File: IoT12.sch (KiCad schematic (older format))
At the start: 98 parts, among them J1 Conn_01x04_Male, Q1 2N7002, Q2 2N7002, Q3 AOD403, SW1 Rotary encoder EC11 Plum 15mm, U1 MAX809S, U2 AT24C32, U3 INA826AID, U4 INA826AID, U5 ADS1115IDGS, U6 LM393, U7 74HC125, U8 LM2596S-ADJ

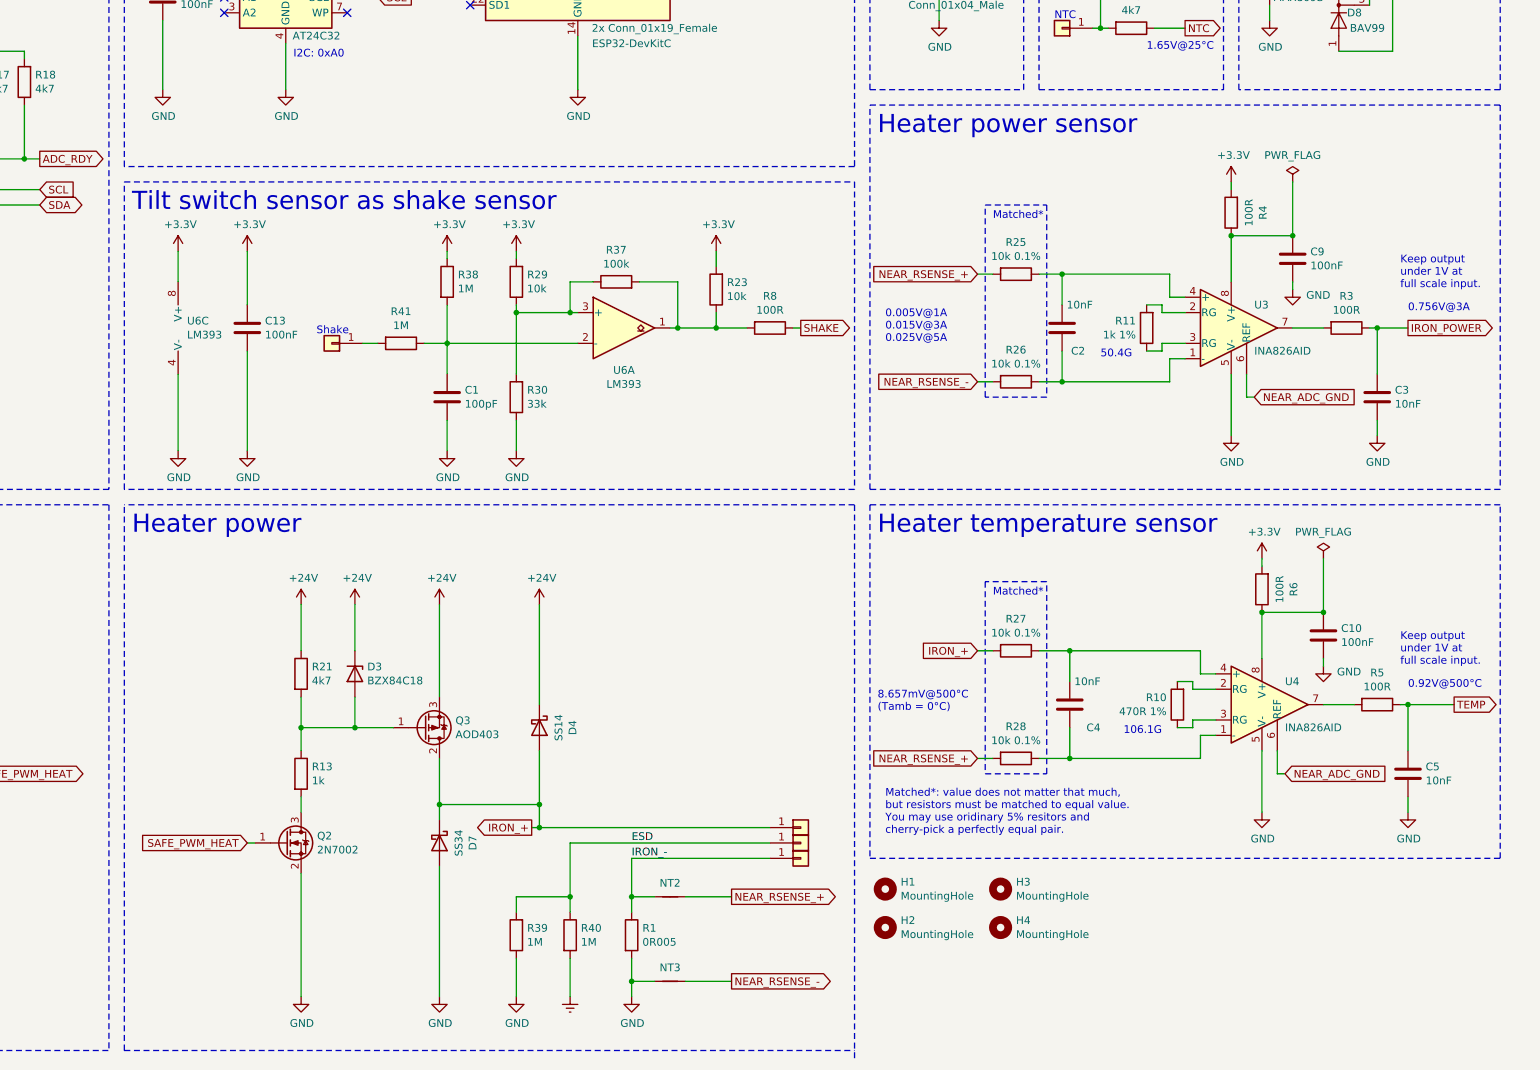
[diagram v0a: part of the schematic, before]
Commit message: Updated schematic and pcb.
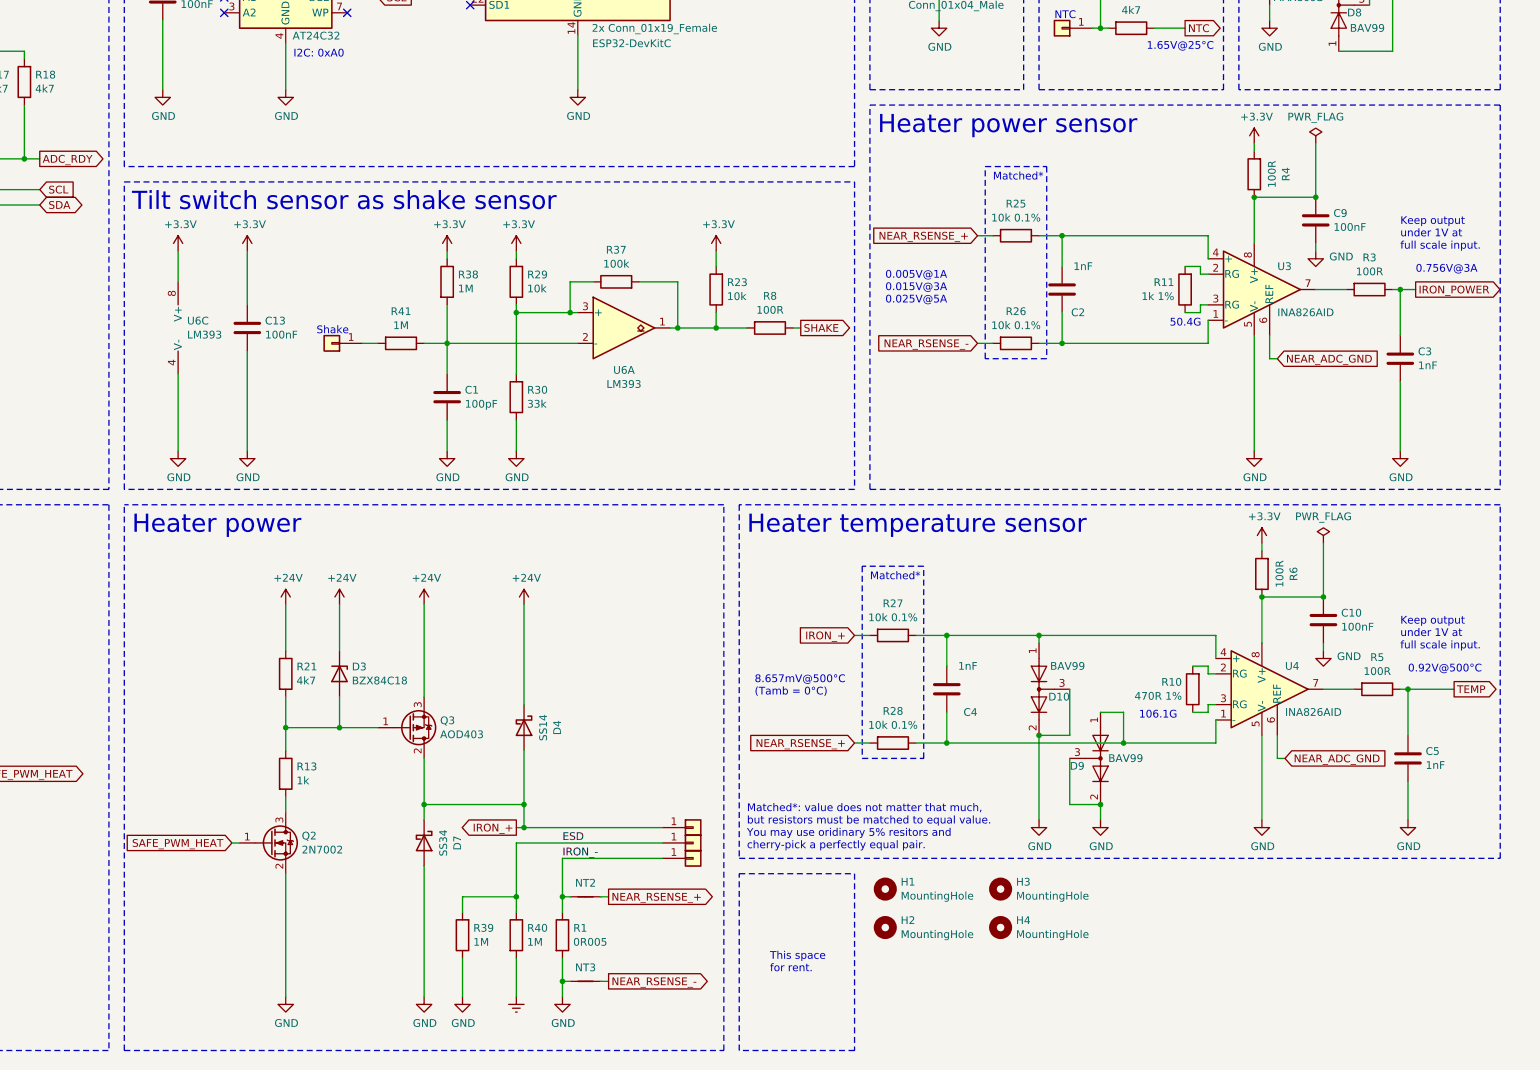
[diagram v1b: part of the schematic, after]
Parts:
- added D10, D9: BAV99, Package_TO_SOT_SMD:SOT-23, symbol Diode:BAV99
- C2, C3, C4, C5: value 10nF -> 1nF
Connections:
- net GND: now also D10.2 (A), D10.3 (K), D9.2 (A), D9.3 (K)
- net at C4.2, R28.1, U4.1 (-): now also D9.1 (K)
- net at C4.1, R27.1, U4.4 (+): now also D10.1 (K)
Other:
- note added: "This space \nfor rent."
- moved on the sheet: C10, C2, C3, C4, C5, C9, D3, D4, D7, NT2, NT3, Q2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
